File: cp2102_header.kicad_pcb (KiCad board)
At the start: 2 copper layers, 15.2 x 22.9 mm, 32 parts, among them J1 FTDI, J2 USB_B_Micro, J22 USB_B_Micro, J8 mount, Q3 BSS138PS, Q4 BSS138PS, U2 CP2102N

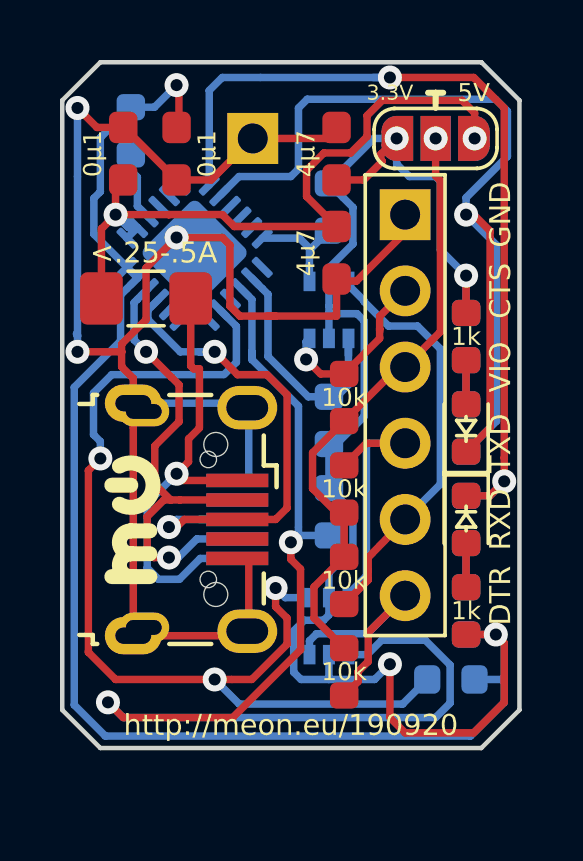
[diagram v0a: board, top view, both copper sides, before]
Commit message: compact dimensions
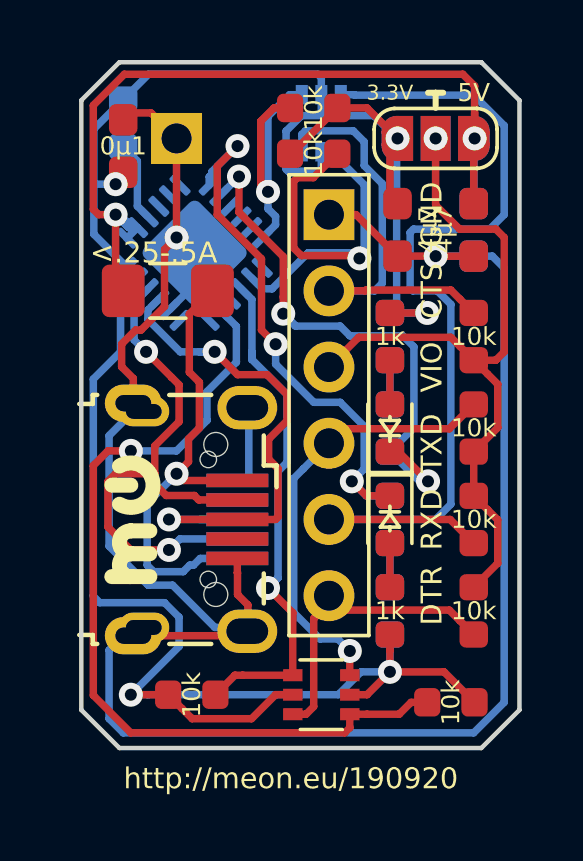
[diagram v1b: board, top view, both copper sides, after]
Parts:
- C24: moved to B.Cu
- Q3, R31, R34, R41, R44: moved to F.Cu
- moved C24 12.0 mm to (91.2, 76.7), turned to 270 degrees
- moved R44 8.90 mm to (85.9, 74.2), turned to 180 degrees
- moved R31 7.62 mm to (81.8, 92.2), turned to 180 degrees
- moved Q4 6.23 mm to (86.1, 73.2)
- moved R46 4.77 mm to (91.2, 80.3)
- moved R33 4.77 mm to (91.2, 89.4)
- moved R36 4.77 mm to (91.2, 83.3)
- moved R43 4.77 mm to (91.2, 86.4)
- moved C23 4.64 mm to (91.2, 76.7)
- moved R41 3.34 mm to (85.9, 72.6), turned to 0 degrees
- moved C21 3.25 mm to (88.6, 76.7), turned to 270 degrees
- moved D21 2.54 mm to (88.4, 83.3)
- moved D22 2.54 mm to (88.4, 86.4)
- moved D23 2.54 mm to (88.4, 83.3)
- moved D24 2.54 mm to (88.4, 86.4)
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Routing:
- net U_TXD: track 39.2 -> 17.7 mm, vias 2 -> 1
- net RXD: track 13.9 -> 31.7 mm
- net TXL: track 33.5 -> 18.4 mm, vias 1 -> 3
- net +3V3: track 94.0 -> 80.1 mm
- net GND: track 61.7 -> 74.1 mm, vias 3 -> 2
- net RXL: track 29.3 -> 18.8 mm, vias 2 -> 3
- net CTS: track 5.89 -> 14.9 mm, vias 1 -> 0
- net U_RXD: track 8.37 -> 14.6 mm, vias 0 -> 1
- net U_DTR: track 34.6 -> 28.7 mm, vias 3 -> 1
- net TXD: track 8.97 -> 14.7 mm, vias 0 -> 1
- net U_CTS: track 3.71 -> 9.44 mm, vias 0 -> 1
- net +5V: track 24.6 -> 29.8 mm
- net VIO: track 20.6 -> 24.3 mm
- net D-: track 16.9 -> 19.8 mm
- net DTR: track 8.44 -> 10.1 mm
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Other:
- board size 15.2 x 22.9 mm -> 14.6 x 22.9 mm
